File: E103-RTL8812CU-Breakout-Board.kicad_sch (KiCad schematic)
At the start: 0 parts

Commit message: board done
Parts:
- added C1, C2: 10u, Capacitor_SMD:C_0805_2012Metric_Pad1.18x1.45mm_HandSolder, symbol Device:C
- added C3, C4: 1u, Capacitor_SMD:C_0805_2012Metric_Pad1.18x1.45mm_HandSolder, symbol Device:C
- added J1, J2: USB_C_Receptacle_USB2.0_16P, Connector_USB:USB_C_Receptacle_GCT_USB4105-xx-A_16P_TopMnt_Horizontal, symbol Connector:USB_C_Receptacle_USB2.0_16P
- added R1, R3, R4, R5: 5.1k, Resistor_SMD:R_0805_2012Metric, symbol Device:R_Small
- added R2: 0, Resistor_SMD:R_0805_2012Metric, symbol Device:R_Small
- added TP1, TP2, TP3, TP4: Clip On, Connector_PinSocket_2.54mm:PinSocket_1x01_P2.54mm_Vertical, symbol Connector:TestPoint
- added TP5, TP6, TP7: Pin, Connector_PinSocket_2.54mm:PinSocket_1x01_P2.54mm_Vertical, symbol Connector:TestPoint
- added U1: Buck_Converter_3.3V, HPRC_Modules:AKEYSRC 3.3V Buck Converter, symbol HPRC_Modules:Buck_Converter_3.3V
- added U2: E103-RTL8812CU, HPRC_Modules:E103-RTL8812CU, symbol HPRC_Modules:E103-RTL8812CU
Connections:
- new net: J1.B5 (CC2), R5.1
- new net: J2.A4 (VBUS), J2.A9 (VBUS), J2.B4 (VBUS), J2.B9 (VBUS), R2.2
- new net: J1.A5 (CC1), R1.1
- new net: TP7.1, U2.17 (RESET)
- new net: U2.10 (NC), U2.11 (NC), U2.12 (NC), U2.2 (NC), U2.7 (NC)
- new net +3.3V: C2.1, C3.1, C4.1, TP5.1, U1.2 (OUT), U2.16 (VDD)
- new net CC1: J2.A5 (CC1), R3.2
- new net CC2: J2.B5 (CC2), R4.2
- new net GND: C1.2, C2.2, C3.2, C4.2, J1.A1 (GND), J1.A12 (GND), J1.B1 (GND), J1.B12 (GND), J1.SH (SHIELD), J2.A1 (GND), J2.A12 (GND), J2.B1 (GND), J2.B12 (GND), J2.SH (SHIELD), R1.2, R3.1, R4.1, R5.2, TP3.1, TP4.1, TP6.1, U1.3 (GND), U1.4 (GND), U2.1 (GND), U2.13 (GND), U2.3 (GND), U2.4 (GND), U2.5 (GND), U2.6 (GND), U2.8 (GND), U2.9 (GND)
- new net USB +: J2.A6 (D+), J2.B6 (D+), U2.15 (DP)
- new net USB -: J2.A7 (D-), J2.B7 (D-), U2.14 (DM)
- new net V_IN: C1.1, J1.A4 (VBUS), J1.A9 (VBUS), J1.B4 (VBUS), J1.B9 (VBUS), R2.1, TP1.1, TP2.1, U1.1 (IN)
- no-connect marks 0 -> 8

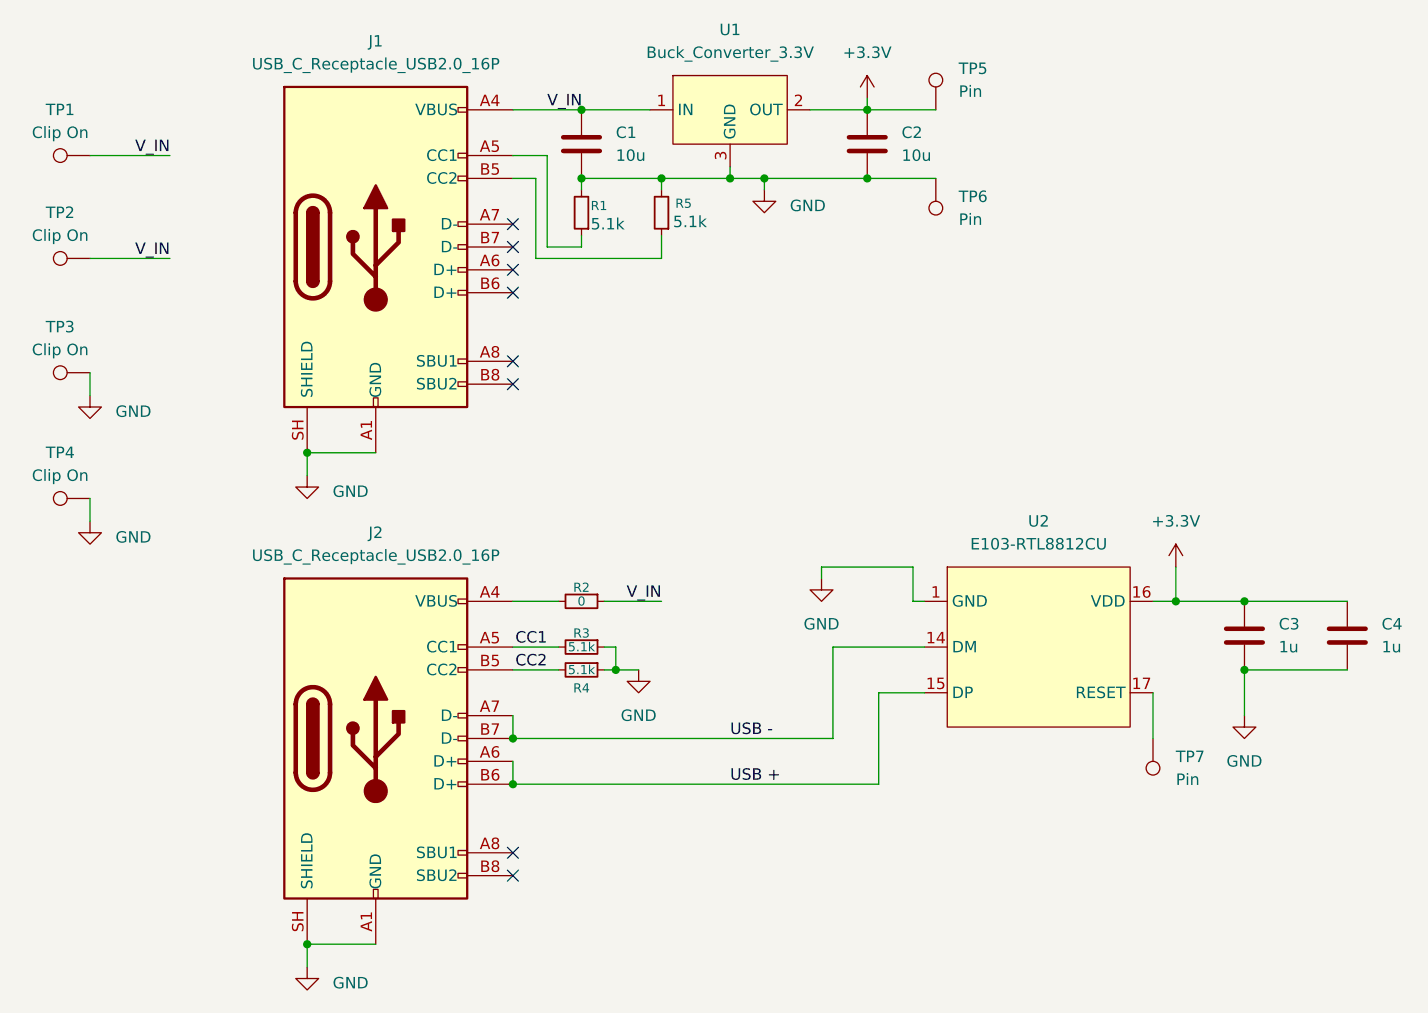
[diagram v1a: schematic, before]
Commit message: boards ordered
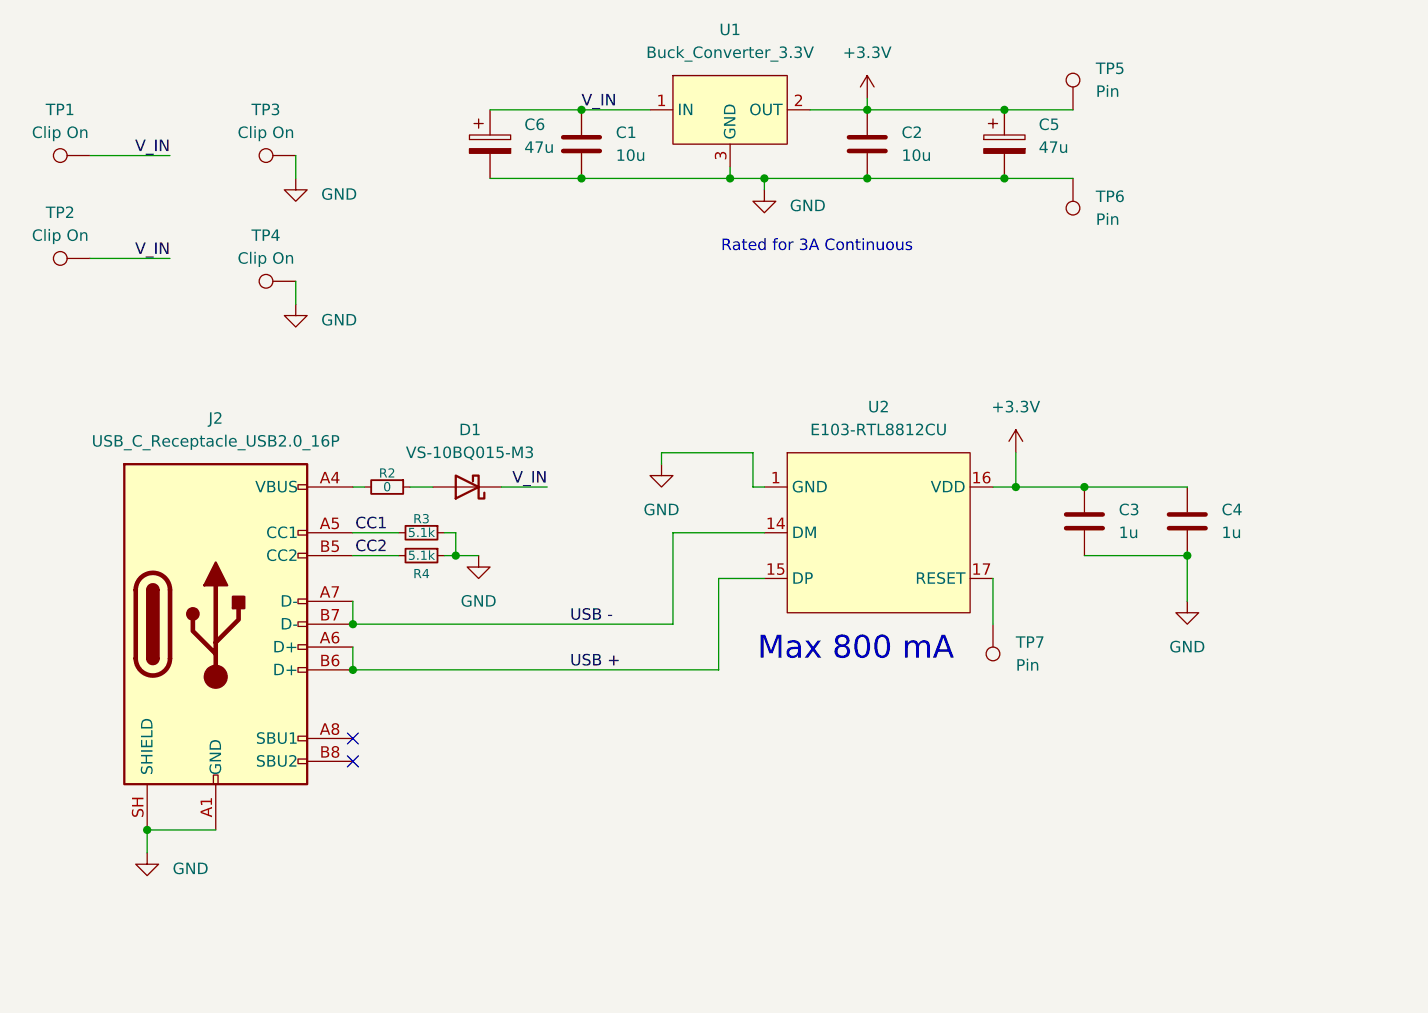
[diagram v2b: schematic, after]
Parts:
- removed J1: USB_C_Receptacle_USB2.0_16P, Connector_USB:USB_C_Receptacle_GCT_USB4105-xx-A_16P_TopMnt_Horizontal, symbol Connector:USB_C_Receptacle_USB2.0_16P
- removed R1, R5: 5.1k, Resistor_SMD:R_0805_2012Metric, symbol Device:R_Small
- added C5, C6: 47u, Capacitor_THT:CP_Radial_D5.0mm_P2.00mm, symbol Device:C_Polarized
- added D1: VS-10BQ015-M3, Diode_SMD:D_SMB_Handsoldering, symbol Device:D_Schottky
- R3, R4: footprint Resistor_SMD:R_0805_2012Metric -> Resistor_SMD:R_0402_1005Metric
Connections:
- net +3.3V: now also C5.1
- net GND: now also C5.2, C6.2
- net V_IN: now also C6.1, D1.1 (K); no longer R2.1
- new net: D1.2 (A), R2.1
- no-connect marks 8 -> 2
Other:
- note added: "Max 800 mA"
- note added: "Rated for 3A Continuous"
- title: (none) -> E103-RTL8812CU Breakout
- moved on the sheet: C3, C4, J2, R2, R3, R4, TP3, TP4, TP5, TP6, TP7, U2
